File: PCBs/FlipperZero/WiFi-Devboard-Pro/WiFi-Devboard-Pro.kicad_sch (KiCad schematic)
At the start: 26 parts

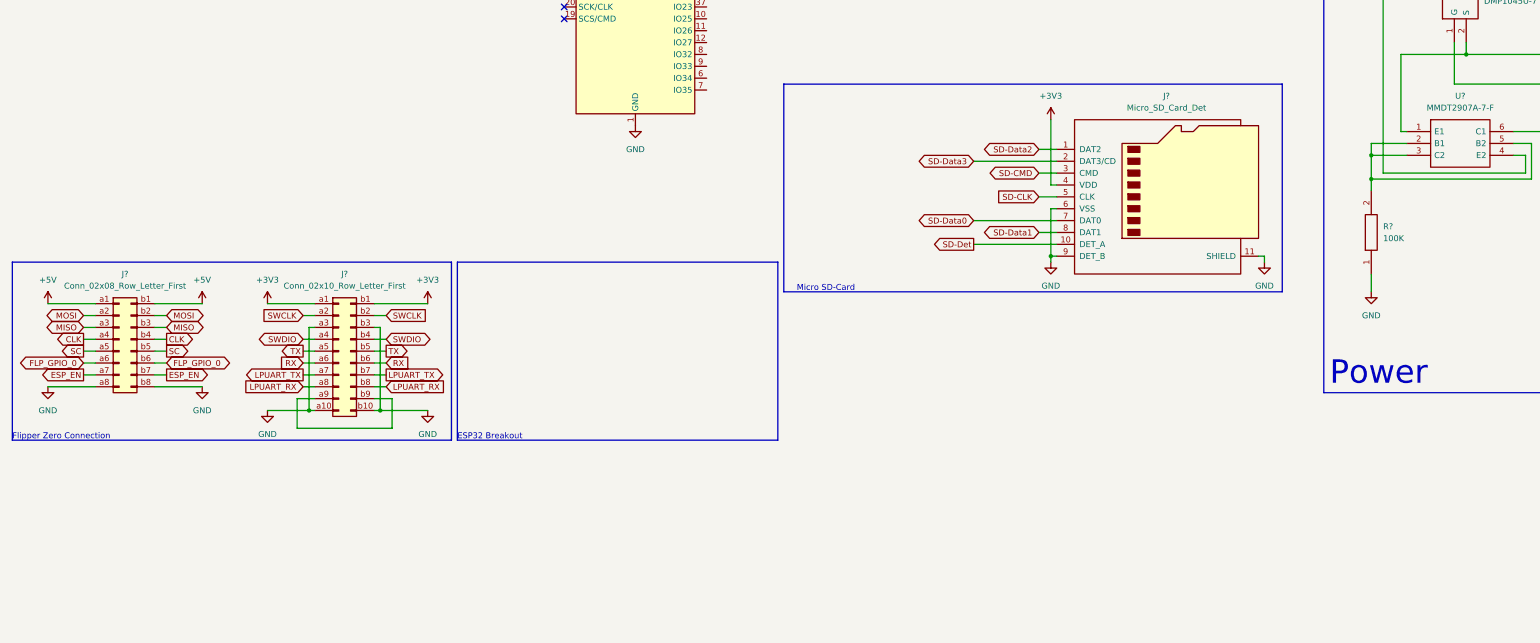
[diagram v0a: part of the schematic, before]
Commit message: add libs, update schematics
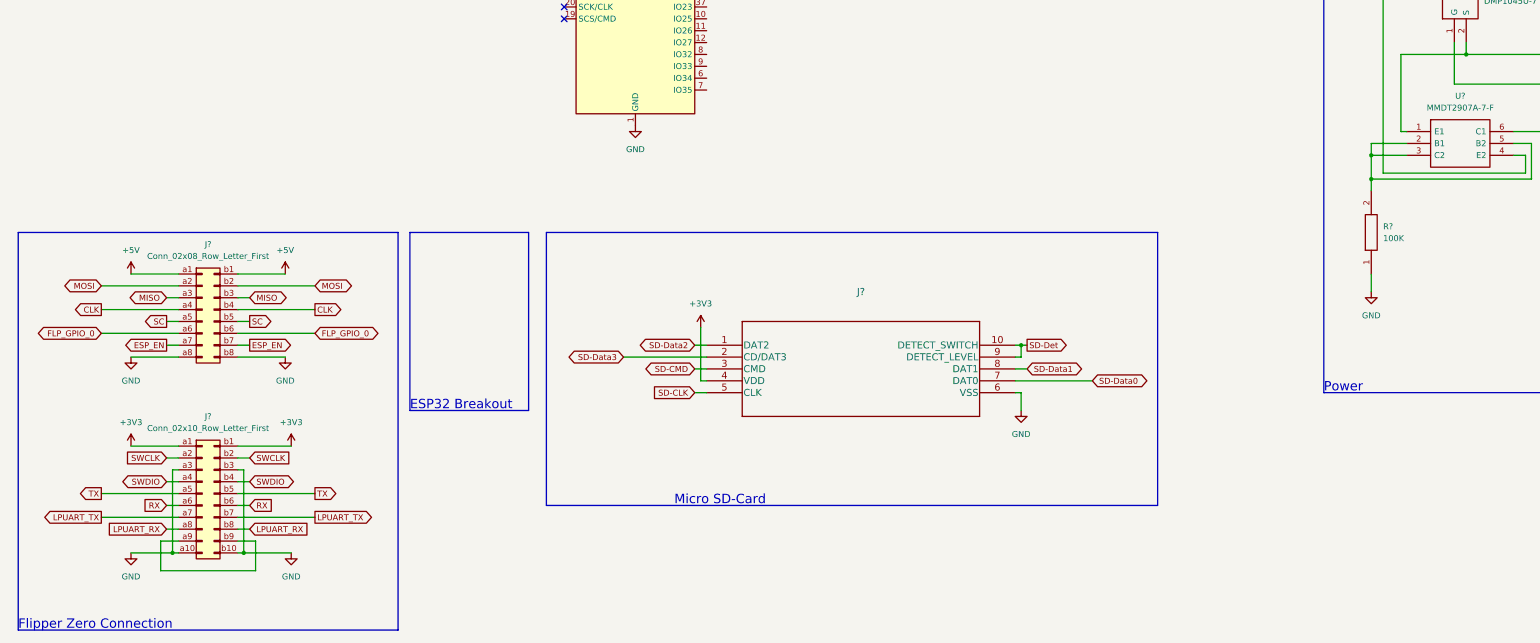
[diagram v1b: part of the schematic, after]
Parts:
- removed J?: Micro_SD_Card_Det, Connector_Card:microSD_HC_Hirose_DM3D-SF, symbol Connector:Micro_SD_Card_Det
- added J?: (no value), symbol 5033981892:5033981892
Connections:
- net +3V3: now also J?.4 (VDD)
- net GND: now also J?.6 (VSS)
- net SD-CLK: now also J?.5 (CLK)
- net SD-CMD: now also J?.3 (CMD)
- net SD-Data0: now also J?.7 (DAT0)
- net SD-Data1: now also J?.8 (DAT1)
- net SD-Data2: now also J?.1 (DAT2)
- net SD-Data3: now also J?.2 (CD/DAT3)
- net SD-Det: now also J?.10 (DETECT_SWITCH), J?.9 (DETECT_LEVEL)
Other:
- moved on the sheet: J?
